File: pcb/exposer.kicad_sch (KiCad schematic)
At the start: 10 parts, among them IC1 ULN2065B, J1 Conn_01x04_Female, J2 Conn_01x02, SW1 SW_Push, SW2 SW_Push, SW3 SW_Push, SW4 SW_SPST

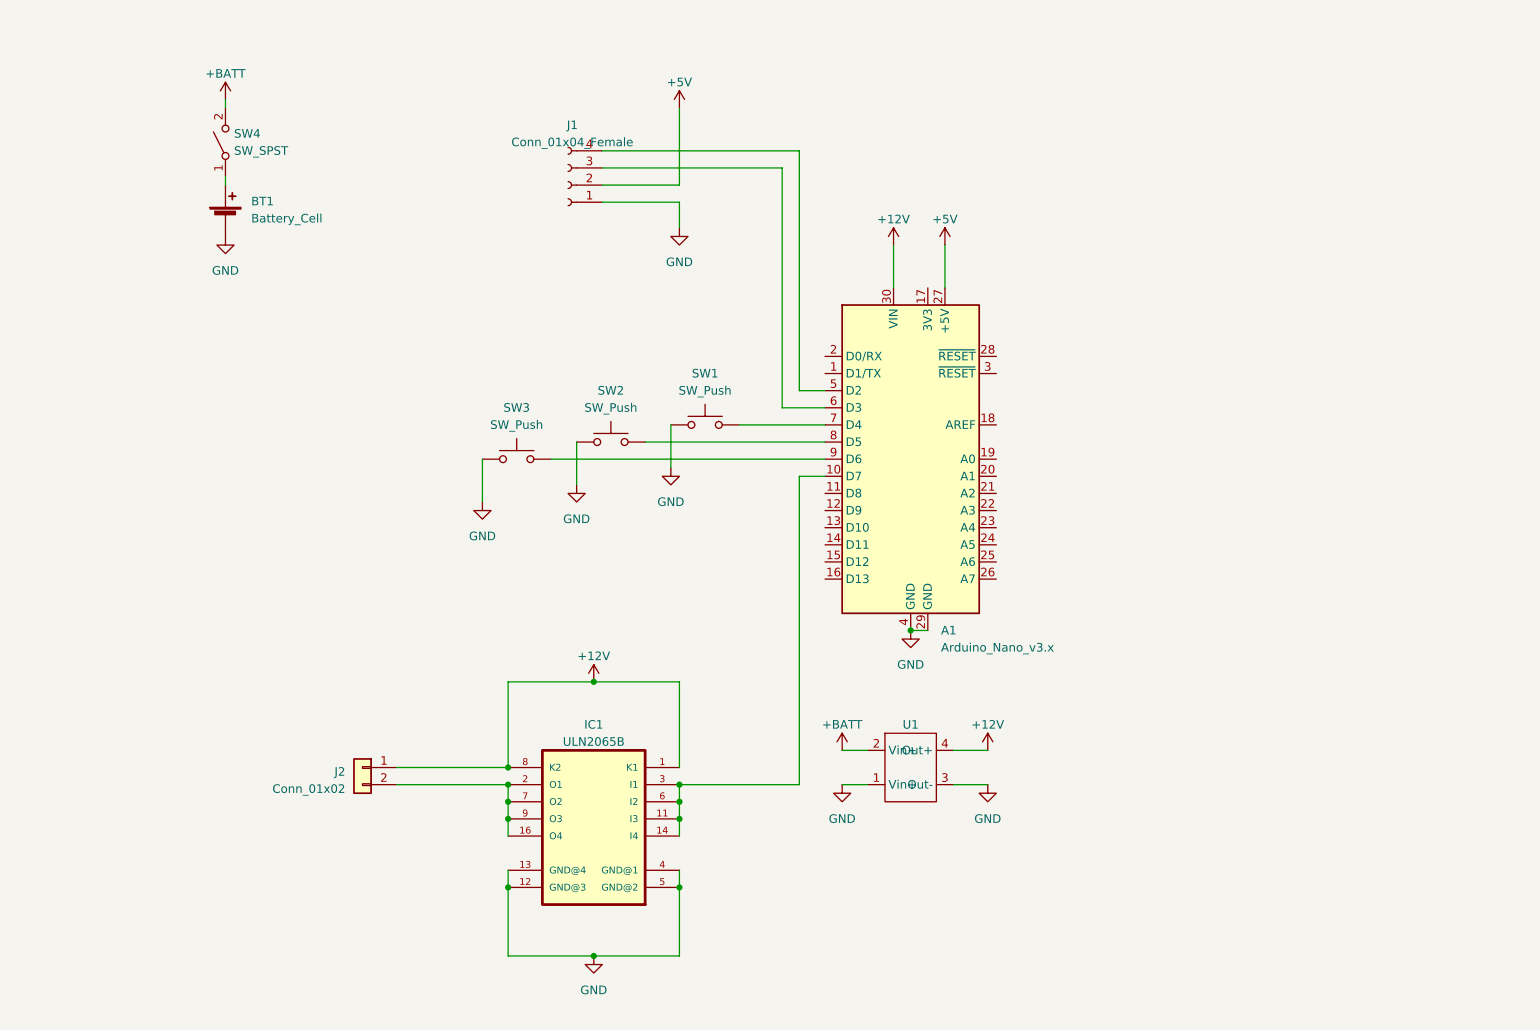
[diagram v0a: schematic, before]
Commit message: yet another exposer
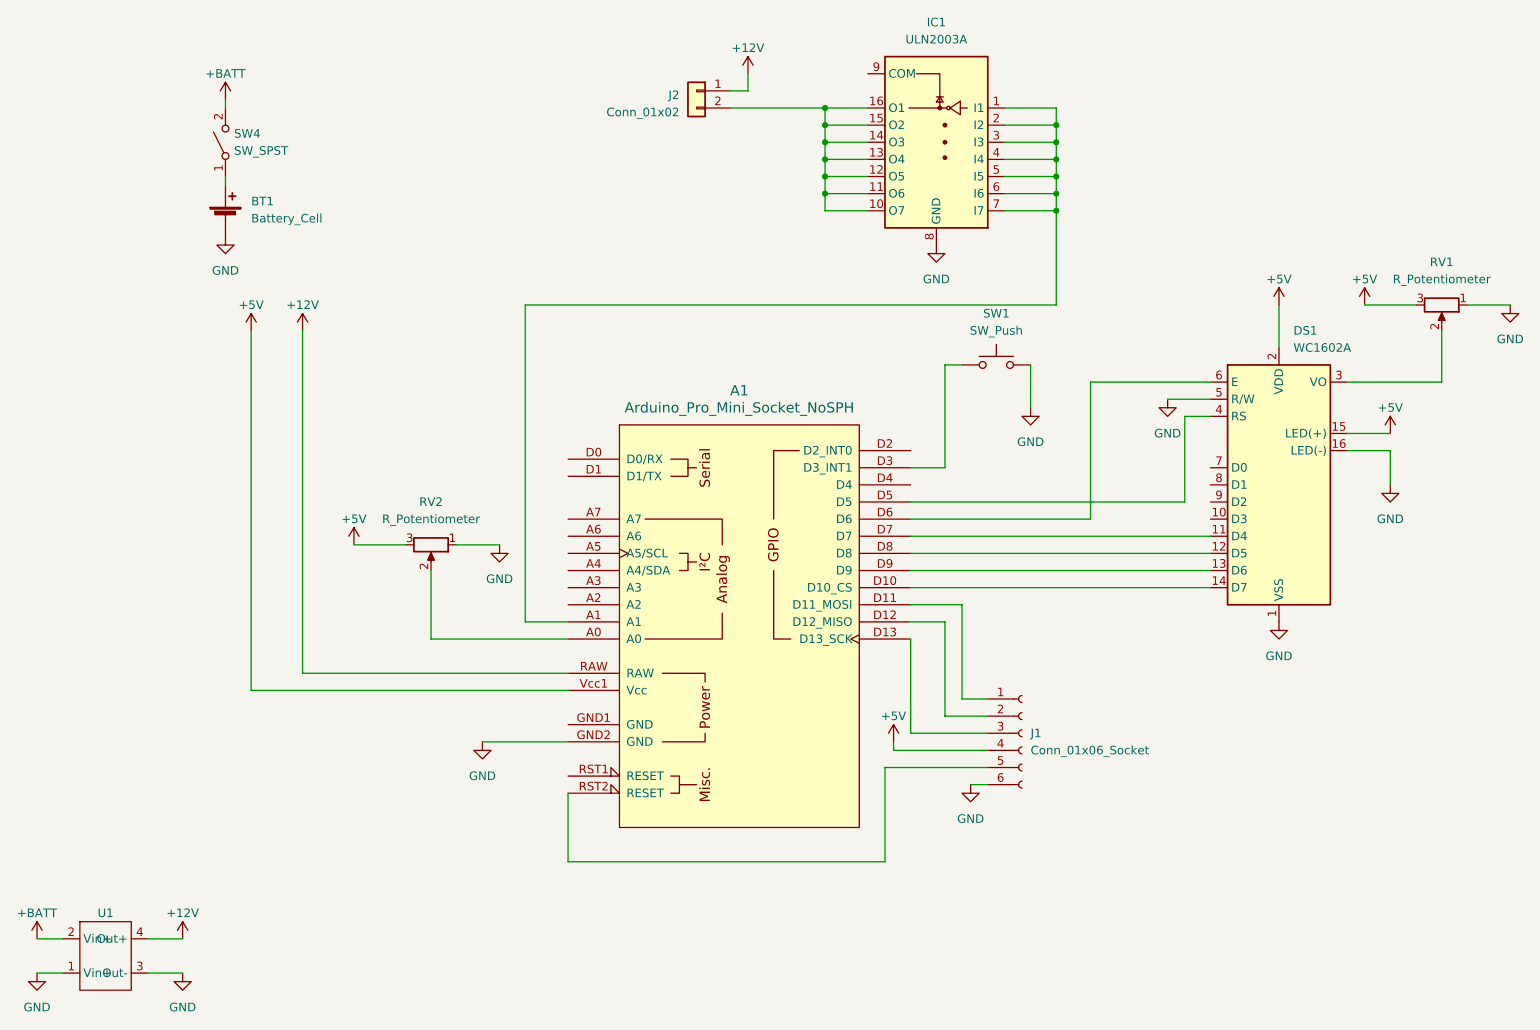
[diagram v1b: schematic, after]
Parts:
- removed A1: Arduino_Nano_v3.x, Module:Arduino_Nano, symbol MCU_Module:Arduino_Nano_v3.x
- removed J1: Conn_01x04_Female, Connector_PinSocket_2.54mm:PinSocket_1x04_P2.54mm_Vertical, symbol Connector:Conn_01x04_Female
- removed SW2, SW3: SW_Push, Button_Switch_THT:SW_PUSH_6mm_H5mm, symbol Switch:SW_Push
- added A1: Arduino_Pro_Mini_Socket_NoSPH, arduino-library:Clone_Pro_Mini_Socket_NoSPH, symbol arduino-library:Arduino_Pro_Mini_Socket_NoSPH
- added DS1: WC1602A, Display:WC1602A, symbol Display_Character:WC1602A
- added J1: Conn_01x06_Socket, Connector_PinSocket_2.54mm:PinSocket_1x06_P2.54mm_Vertical, symbol Connector:Conn_01x06_Socket
- added RV1: R_Potentiometer, Potentiometer_THT:Potentiometer_ACP_CA6-H2,5_Horizontal, symbol Device:R_Potentiometer
- added RV2: R_Potentiometer, Potentiometer_THT:Potentiometer_Alps_RK163_Single_Horizontal, symbol Device:R_Potentiometer
- BT1: footprint Battery:BatteryHolder_Keystone_1042_1x18650 -> Battery:BatteryHolder_MPD_BH-18650-PC
- IC1: value ULN2065B -> ULN2003A; symbol ULN2065B:ULN2065B -> Transistor_Array:ULN2003A
- SW4: footprint Connector_Molex:Molex_Micro-Fit_3.0_43650-0315_1x03_P3.00mm_Vertical -> Button_Switch_THT:SW_Slide_SPDT_Straight_CK_OS102011MS2Q
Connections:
- net +12V: now also A1.RAW; no longer IC1.1 (K1), IC1.8 (K2)
- net +5V: now also A1.Vcc1 (Vcc), DS1.15 (LED(+)), DS1.2 (VDD), J1.4 (Pin_4), RV1.3, RV2.3
- net GND: now also IC1.8 (GND), A1.GND2 (GND), DS1.1 (VSS), DS1.16 (LED(-)), DS1.5 (R/W), J1.6 (Pin_6), RV1.1, RV2.1; no longer IC1.12 (GND@3), IC1.13 (GND@4), IC1.4 (GND@1), IC1.5 (GND@2)
- net at SW1.2: now also A1.D3 (D3_INT1)
- net at IC1.3 (I3), IC1.6 (I6): now also IC1.1 (I1), IC1.2 (I2), IC1.4 (I4), IC1.5 (I5), IC1.7 (I7), A1.A1; no longer IC1.11 (I3), IC1.14 (I4)
- new net: A1.D11 (D11_MOSI), J1.1 (Pin_1)
- new net: A1.D12 (D12_MISO), J1.2 (Pin_2)
- new net: A1.D13 (D13_SCK), J1.3 (Pin_3)
- new net: A1.RST2 (RESET), J1.5 (Pin_5)
- new net: DS1.3 (VO), RV1.2
- new net: IC1.10 (O7), IC1.11 (O6), IC1.12 (O5), IC1.13 (O4), IC1.14 (O3), IC1.15 (O2), IC1.16 (O1), J2.2 (Pin_2)
- new net: A1.A0, RV2.2
- new net: A1.D10 (D10_CS), DS1.14 (D7)
- new net: A1.D5, DS1.4 (RS)
- new net: A1.D6, DS1.6 (E)
- new net: A1.D7, DS1.11 (D4)
- new net: A1.D8, DS1.12 (D5)
- new net: A1.D9, DS1.13 (D6)
- now unconnected: IC1.9 (O3)
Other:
- moved on the sheet: J2, SW1, U1
